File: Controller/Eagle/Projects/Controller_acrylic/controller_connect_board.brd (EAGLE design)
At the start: 185 x 33 mm, 13 parts, among them J1 JST_3PIN_GND_VDD_SIG, J2 JST_3PIN_GND_VDD_SIG, J3 JST_3PIN_GND_VDD_SIG, J4 JST_3PIN_GND_VDD_SIG, J5 GIMBAL_3PIN_MATCH_TDOCU

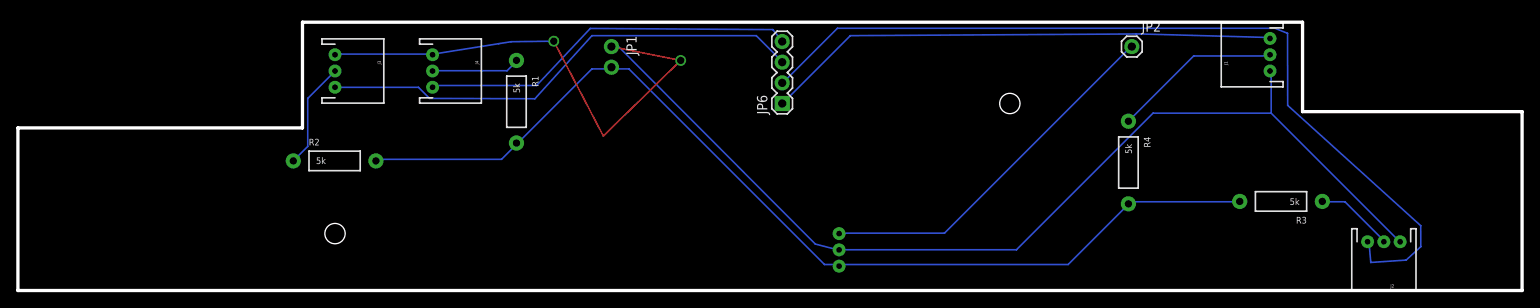
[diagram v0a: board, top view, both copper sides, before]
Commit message: FORGOT THE BUTTON WOW WOW I...WOW
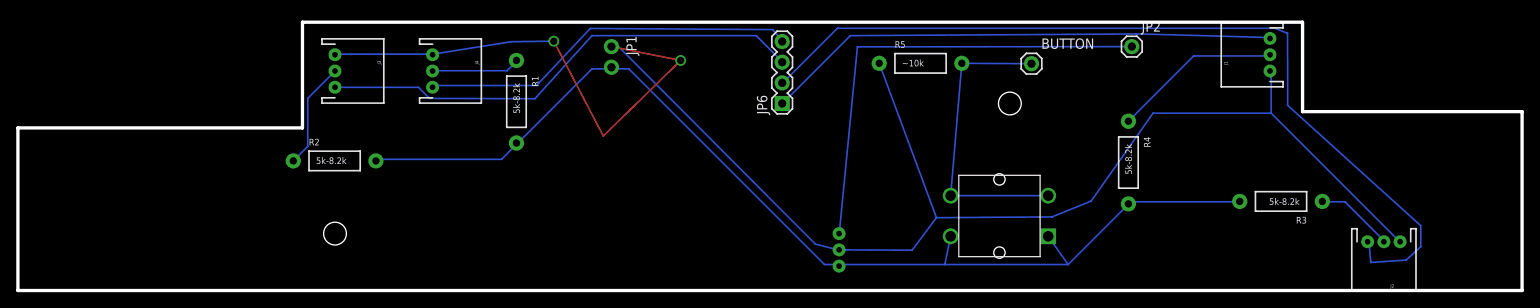
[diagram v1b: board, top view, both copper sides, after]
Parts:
- added BUTTON: (no value), SparkFun-Connectors:1X01
- added R5: ~10k, SparkFun-Resistors:AXIAL-0.4
- added U$2: BUTTON-TACTILE-SQUARE, Controller:BUTTON-TACTILE-SQUARE-ADAFRUIT1010
- R1, R2, R3, R4: value 5k -> 5k-8.2k
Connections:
- new net N$6: BUTTON.1, R5.P$2, U$2.S, U$2.S2
- net 3.3V: now also U$2.P, U$2.P2
- net GND: now also R5.P$1
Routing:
- net N$6: track 0.00 -> 36.9 mm
- net GND: track 188.1 -> 209.4 mm
- net N$9: track 45.5 -> 56.9 mm
- net 3.3V: track 124.8 -> 132.6 mm
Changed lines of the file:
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@@
 <element name="J3" library="Controller" package="JST-3-PTH-REVERSE" value="JST_3PIN_GND_VDD_SIG" x="71" y="49" rot="R270"/>
 <element name="J4" library="Controller" package="JST-3-PTH-REVERSE" value="JST_3PIN_GND_VDD_SIG" x="83" y="49" rot="R270"/>
-<element name="R1" library="SparkFun-Resistors" package="AXIAL-0.4" value="5k" x="93.318003125" y="45.219046875" rot="R270"/>
-<element name="R2" library="SparkFun-Resistors" package="AXIAL-0.4" value="5k" x="70.949403125" y="37.939940625"/>
-<element name="R3" library="SparkFun-Resistors" package="AXIAL-0.4" value="5k" x="187.352325" y="32.957490625" rot="R180"/>
-<element name="R4" library="SparkFun-Resistors" package="AXIAL-0.4" value="5k" x="168.58266875" y="37.739028125" rot="R270"/>
+<element name="R1" library="SparkFun-Resistors" package="AXIAL-0.4" value="5k-8.2k" x="93.318003125" y="45.219046875" rot="R270"/>
+<element name="R2" library="SparkFun-Resistors" package="AXIAL-0.4" value="5k-8.2k" x="70.949403125" y="37.939940625"/>
+<element name="R3" library="SparkFun-Resistors" package="AXIAL-0.4" value="5k-8.2k" x="187.352325" y="32.957490625" rot="R180"/>
+<element name="R4" library="SparkFun-Resistors" package="AXIAL-0.4" value="5k-8.2k" x="168.58266875" y="37.739028125" rot="R270"/>
 <element name="JP6" library="SparkFun-Connectors" package="1X04" value="" x="126" y="45" rot="R90"/>
 <element name="JP1" library="SparkFun-Connectors" package="1X02_NO_SILK" value="" x="105" y="52" rot="R270"/>
@@
 <element name="JP2" library="SparkFun-Connectors" package="1X01" value="" x="169" y="52"/>
 <element name="U$1" library="Controller" package="CONNECTOR_BOARD_OUTLINE" value="" x="0" y="0"/>
+<element name="U$2" library="Controller" package="BUTTON-TACTILE-SQUARE-ADAFRUIT1010" value="BUTTON-TACTILE-SQUARE" x="152.719" y="31.166" rot="R180"/>
+<element name="BUTTON" library="SparkFun-Connectors" package="1X01" value="" x="156.66" y="49.897"/>
+<element name="R5" library="SparkFun-Resistors" package="AXIAL-0.4" value="~10k" x="143.013" y="49.942"/>
 </elements>
 <signals>
@@
 <wire x1="82.855" y1="51.075" x2="83" y2="51" width="0.2" layer="16"/>
 <wire x1="130.071" y1="27.715" x2="132.795" y2="27.013" width="0.2" layer="16"/>
-<wire x1="105.968" y1="51.9" x2="130.071" y2="27.715" width="0.2" layer="16"/>
+<wire x1="105.968" y1="51.9" x2="122.40503125" y2="35.40705" width="0.2" layer="16"/>
+<wire x1="122.40503125" y1="35.40705" x2="130.071" y2="27.715" width="0.2" layer="16"/>
 <wire x1="132.795" y1="27.013" x2="133" y2="27" width="0.2" layer="16"/>
 <wire x1="105.968" y1="51.9" x2="105" y2="52" width="0.2" layer="16"/>
@@
 <wire x1="83.082" y1="51.075" x2="83" y2="51" width="0.2" layer="16"/>
 <wire x1="171.612" y1="43.811" x2="186.14" y2="43.811" width="0.2" layer="16"/>
-<wire x1="154.814" y1="27.013" x2="171.612" y2="43.811" width="0.2" layer="16"/>
-<wire x1="133.022" y1="27.013" x2="154.814" y2="27.013" width="0.2" layer="16"/>
 <wire x1="133.022" y1="27.013" x2="133" y2="27" width="0.2" layer="16"/>
 <via x="97.909" y="52.665" extent="1-16" drill="0.9"/>
@@
 <wire x1="97.909" y1="52.665" x2="104" y2="41" width="0.2" layer="1"/>
 <wire x1="104" y1="41" x2="113.515" y2="50.296" width="0.2" layer="1"/>
+<contactref element="R5" pad="P$1"/>
+<wire x1="171.612" y1="43.811" x2="164" y2="33" width="0.2" layer="16"/>
+<wire x1="164" y1="33" x2="159.184" y2="31.052" width="0.2" layer="16"/>
+<wire x1="159.184" y1="31.052" x2="144.977" y2="30.956" width="0.2" layer="16"/>
+<wire x1="144.977" y1="30.956" x2="141.977" y2="26.96" width="0.2" layer="16"/>
+<wire x1="141.977" y1="26.96" x2="133" y2="27" width="0.2" layer="16"/>
+<wire x1="144.977" y1="30.956" x2="137.933" y2="49.942" width="0.2" layer="16"/>
 </signal>
 <signal name="N$1">
@@
 <wire x1="104.874" y1="49.259" x2="105" y2="49.46" width="0.2" layer="16"/>
 <wire x1="93.524" y1="40.179" x2="93.318003125" y2="40.139046875" width="0.2" layer="16"/>
-<wire x1="161.17" y1="25.197" x2="133.022" y2="25.197" width="0.2" layer="16"/>
+<wire x1="161.17" y1="25.197" x2="146" y2="25.197" width="0.2" layer="16"/>
+<wire x1="146" y1="25.197" x2="133.022" y2="25.197" width="0.2" layer="16"/>
 <wire x1="168.434" y1="32.461" x2="161.17" y2="25.197" width="0.2" layer="16"/>
 <wire x1="133.022" y1="25.197" x2="133" y2="25" width="0.2" layer="16"/>
@@
 <wire x1="105.101" y1="49.259" x2="105" y2="49.46" width="0.2" layer="16"/>
 <wire x1="132.795" y1="25.197" x2="133" y2="25" width="0.2" layer="16"/>
+<contactref element="U$2" pad="P2"/>
+<wire x1="146.719" y1="28.666" x2="146" y2="25.197" width="0.2" layer="16"/>
+<contactref element="U$2" pad="P"/>
+<wire x1="161.17" y1="25.197" x2="158.719" y2="28.666" width="0.2" layer="16"/>
 </signal>
 <signal name="PITCH">
@@
 <contactref element="J5" pad="3"/>
 <contactref element="JP2" pad="1"/>
-<wire x1="145.961" y1="29.056" x2="133.022" y2="29.056" width="0.2" layer="16"/>
-<wire x1="168.888" y1="51.983" x2="145.961" y2="29.056" width="0.2" layer="16"/>
 <wire x1="133.022" y1="29.056" x2="133" y2="29" width="0.2" layer="16"/>
 <wire x1="168.888" y1="51.983" x2="169" y2="52" width="0.2" layer="16"/>
+<wire x1="133.022" y1="29.056" x2="135.253" y2="51.966" width="0.2" layer="16"/>
+<wire x1="135.253" y1="51.966" x2="169" y2="52" width="0.2" layer="16"/>
+</signal>
+<signal name="N$6">
+<contactref element="U$2" pad="S2"/>
+<contactref element="BUTTON" pad="1"/>
+<contactref element="R5" pad="P$2"/>
+<wire x1="156.66" y1="49.897" x2="148.093" y2="49.942" width="0.2" layer="16"/>
+<wire x1="148.093" y1="49.942" x2="146.719" y2="33.666" width="0.2" layer="16"/>
+<contactref element="U$2" pad="S"/>
+<wire x1="146.719" y1="33.666" x2="158.719" y2="33.666" width="0.2" layer="16"/>
 </signal>
 </signals>
